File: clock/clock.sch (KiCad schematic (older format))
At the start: 76 parts, among them J1 FTDI, J2 USB, J3 TP, SW1 SW_SPST, SW2 SW_SPST, SW3 SW_SPST, SW4 SW_SPST, SW5 SW_SPST, U1 iv12, U10 PCA9685PW, U11 ATmega328P-AU, U12 DS3231M, U13 MT3608, U2 iv12, U3 iv12, U4 iv12, U5 ULN2003, U6 ULN2003, U7 ULN2003, U8 ULN2003, U9 PCA9685PW, Y1 16MHz

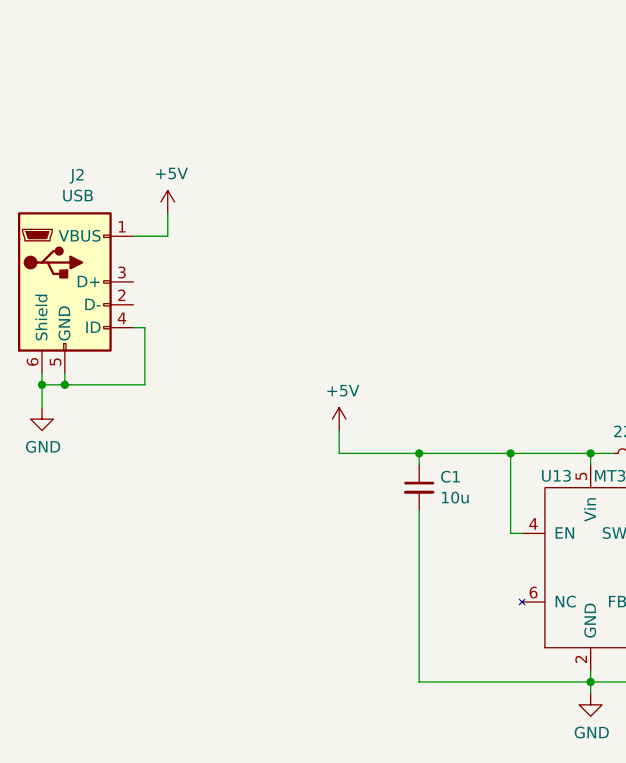
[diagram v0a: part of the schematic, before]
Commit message: More cleanup
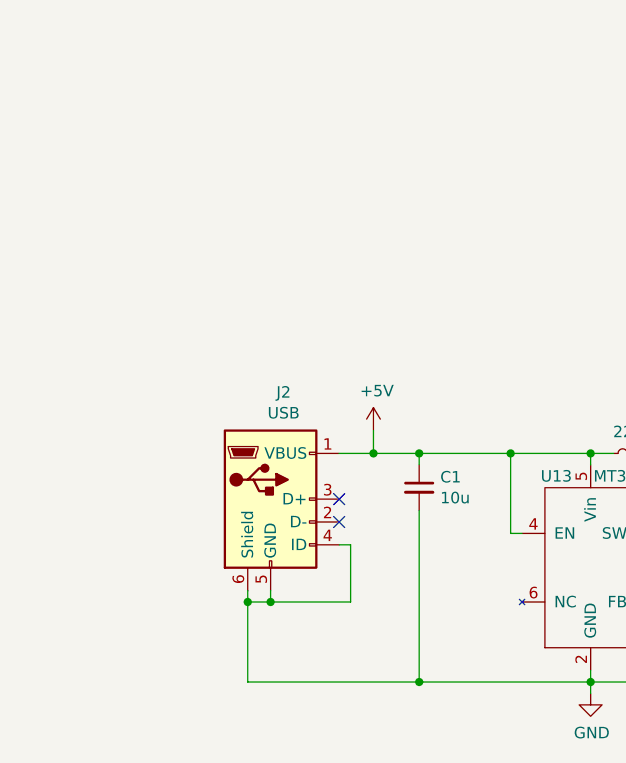
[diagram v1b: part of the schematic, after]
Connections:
- no-connect marks 2 -> 4
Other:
- moved on the sheet: J2
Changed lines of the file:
@@
 L power:+5V #PWR0134
 U 1 1 5D8C47A1
-P 3550 8450
-F 0 "#PWR0134" H 3550 8300 50  0001 C CNN
-F 1 "+5V" H 3565 8623 50  0000 C CNN
-F 2 "" H 3550 8450 50  0001 C CNN
-F 3 "" H 3550 8450 50  0001 C CNN
-	1    3550 8450
+P 3700 8450
+F 0 "#PWR0134" H 3700 8300 50  0001 C CNN
+F 1 "+5V" H 3715 8623 50  0000 C CNN
+F 2 "" H 3700 8450 50  0001 C CNN
+F 3 "" H 3700 8450 50  0001 C CNN
+	1    3700 8450
 	1    0    0    -1
 $EndComp
@@
 	7200 5000 7500 5000
 Wire Wire Line
-	3550 8450 3550 8550
-Wire Wire Line
-	3550 8550 3900 8550
+	3550 8550 3700 8550
 Wire Wire Line
 	7500 5000 7800 5000
@@
 	6250 4850 6150 4850
 $Comp
-L power:GND #PWR0147
-U 1 1 5CD38EBC
-P 2250 8350
-F 0 "#PWR0147" H 2250 8100 50  0001 C CNN
-F 1 "GND" H 2255 8177 50  0000 C CNN
-F 2 "" H 2250 8350 50  0001 C CNN
-F 3 "" H 2250 8350 50  0001 C CNN
-	1    2250 8350
-	1    0    0    -1
-$EndComp
-$Comp
-L power:+5V #PWR0148
-U 1 1 5CD75A01
-P 2800 7500
-F 0 "#PWR0148" H 2800 7350 50  0001 C CNN
-F 1 "+5V" H 2815 7673 50  0000 C CNN
-F 2 "" H 2800 7500 50  0001 C CNN
-F 3 "" H 2800 7500 50  0001 C CNN
-	1    2800 7500
-	1    0    0    -1
-$EndComp
-$Comp
 L clock-rescue:USB_OTG-conn1 J2
 U 1 1 5C6DC8AA
-P 2350 7800
-F 0 "J2" H 2407 8267 50  0000 C CNN
-F 1 "USB" H 2407 8176 50  0000 C CNN
-F 2 "Connector_USB:USB_Micro-B_Molex-105133-0001" H 2500 7750 50  0001 C CNN
-F 3 "" H 2500 7750 50  0001 C CNN
-	1    2350 7800
-	1    0    0    -1
-$EndComp
-Wire Wire Line
-	2650 7600 2800 7600
-Wire Wire Line
-	2800 7600 2800 7500
-Wire Wire Line
-	2250 8200 2250 8250
-Wire Wire Line
-	2250 8250 2350 8250
-Wire Wire Line
-	2350 8250 2350 8200
-Connection ~ 2250 8250
-Wire Wire Line
-	2250 8250 2250 8350
-Wire Wire Line
-	2350 8250 2700 8250
-Wire Wire Line
-	2700 8250 2700 8000
-Wire Wire Line
-	2700 8000 2650 8000
-Connection ~ 2350 8250
+P 3250 8750
+F 0 "J2" H 3307 9217 50  0000 C CNN
+F 1 "USB" H 3307 9126 50  0000 C CNN
+F 2 "Connector_USB:USB_Micro-B_Molex-105133-0001" H 3400 8700 50  0001 C CNN
+F 3 "" H 3400 8700 50  0001 C CNN
+	1    3250 8750
+	1    0    0    -1
+$EndComp
 $Comp
 L Connector:Conn_01x05_Female J3
@@
 Wire Wire Line
 	8950 3200 8950 3250
+Wire Wire Line
+	3150 9150 3150 9200
+Wire Wire Line
+	3150 9550 3900 9550
+Connection ~ 3900 9550
+Wire Wire Line
+	3250 9150 3250 9200
+Wire Wire Line
+	3250 9200 3150 9200
+Connection ~ 3150 9200
+Wire Wire Line
+	3150 9200 3150 9550
+Wire Wire Line
+	3250 9200 3600 9200
+Wire Wire Line
+	3600 9200 3600 8950
+Wire Wire Line
+	3600 8950 3550 8950
+Connection ~ 3250 9200
+NoConn ~ 3550 8750
+NoConn ~ 3550 8850
+Wire Wire Line
+	3700 8450 3700 8550
+Connection ~ 3700 8550
+Wire Wire Line
+	3700 8550 3900 8550
 $EndSCHEMATC
